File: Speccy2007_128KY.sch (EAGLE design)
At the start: 121 parts, among them J1 0, J2 0, X1 5V, X2 SCART-F, X3 PS/2 KB, X3P KB, X4 SD Card, X5 ByteBlaster, X6 AVRISP

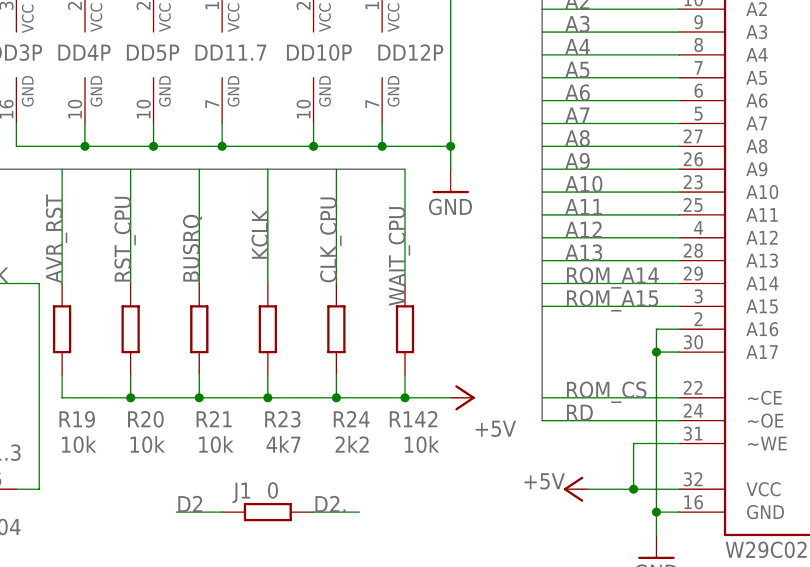
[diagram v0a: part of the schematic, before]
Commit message: t2
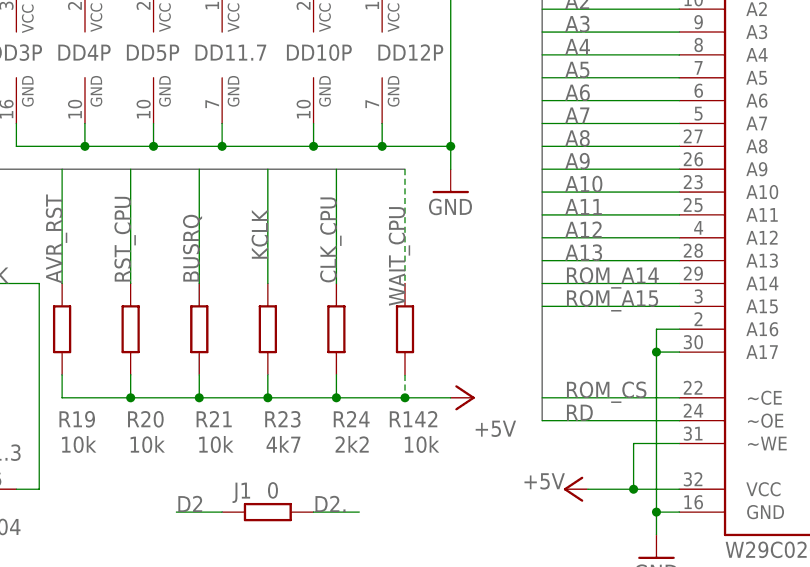
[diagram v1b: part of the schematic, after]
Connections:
- net N$16 renamed CDDAT3
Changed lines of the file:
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@@
 <grid distance="100" unitdist="mil" unit="mil" style="lines" multiple="1" display="yes" altdistance="0.01" altunitdist="inch" altunit="inch"/>
 <layers>
-<layer number="1" name="Top" color="4" fill="1" visible="yes" active="no"/>
-<layer number="2" name="Route2" color="1" fill="3" visible="yes" active="no"/>
-<layer number="3" name="Route3" color="4" fill="3" visible="yes" active="no"/>
-<layer number="4" name="Route4" color="1" fill="4" visible="yes" active="no"/>
-<layer number="5" name="Route5" color="4" fill="4" visible="yes" active="no"/>
-<layer number="6" name="Route6" color="1" fill="8" visible="yes" active="no"/>
-<layer number="7" name="Route7" color="4" fill="8" visible="yes" active="no"/>
-<layer number="8" name="Route8" color="1" fill="2" visible="yes" active="no"/>
-<layer number="9" name="Route9" color="4" fill="2" visible="yes" active="no"/>
-<layer number="10" name="Route10" color="1" fill="7" visible="yes" active="no"/>
-<layer number="11" name="Route11" color="4" fill="7" visible="yes" active="no"/>
-<layer number="12" name="Route12" color="1" fill="5" visible="yes" active="no"/>
-<layer number="13" name="Route13" color="4" fill="5" visible="yes" active="no"/>
-<layer number="14" name="Route14" color="1" fill="6" visible="yes" active="no"/>
-<layer number="15" name="Route15" color="4" fill="6" visible="yes" active="no"/>
-<layer number="16" name="Bottom" color="1" fill="1" visible="yes" active="no"/>
-<layer number="17" name="Pads" color="2" fill="1" visible="yes" active="no"/>
-<layer number="18" name="Vias" color="2" fill="1" visible="yes" active="no"/>
-<layer number="19" name="Unrouted" color="6" fill="1" visible="yes" active="no"/>
-<layer number="20" name="Dimension" color="15" fill="1" visible="yes" active="no"/>
-<layer number="21" name="tPlace" color="7" fill="1" visible="yes" active="no"/>
-<layer number="22" name="bPlace" color="7" fill="1" visible="yes" active="no"/>
-<layer number="23" name="tOrigins" color="15" fill="1" visible="yes" active="no"/>
-<layer number="24" name="bOrigins" color="15" fill="1" visible="yes" active="no"/>
-<layer number="25" name="tNames" color="7" fill="1" visible="yes" active="no"/>
-<layer number="26" name="bNames" color="7" fill="1" visible="yes" active="no"/>
-<layer number="27" name="tValues" color="7" fill="1" visible="yes" active="no"/>
-<layer number="28" name="bValues" color="7" fill="1" visible="yes" active="no"/>
+<layer number="1" name="Top" color="4" fill="1" visible="no" active="no"/>
+<layer number="2" name="Route2" color="1" fill="3" visible="no" active="no"/>
+<layer number="3" name="Route3" color="4" fill="3" visible="no" active="no"/>
+<layer number="4" name="Route4" color="1" fill="4" visible="no" active="no"/>
+<layer number="5" name="Route5" color="4" fill="4" visible="no" active="no"/>
+<layer number="6" name="Route6" color="1" fill="8" visible="no" active="no"/>
+<layer number="7" name="Route7" color="4" fill="8" visible="no" active="no"/>
+<layer number="8" name="Route8" color="1" fill="2" visible="no" active="no"/>
+<layer number="9" name="Route9" color="4" fill="2" visible="no" active="no"/>
+<layer number="10" name="Route10" color="1" fill="7" visible="no" active="no"/>
+<layer number="11" name="Route11" color="4" fill="7" visible="no" active="no"/>
+<layer number="12" name="Route12" color="1" fill="5" visible="no" active="no"/>
+<layer number="13" name="Route13" color="4" fill="5" visible="no" active="no"/>
+<layer number="14" name="Route14" color="1" fill="6" visible="no" active="no"/>
+<layer number="15" name="Route15" color="4" fill="6" visible="no" active="no"/>
+<layer number="16" name="Bottom" color="1" fill="1" visible="no" active="no"/>
+<layer number="17" name="Pads" color="2" fill="1" visible="no" active="no"/>
+<layer number="18" name="Vias" color="2" fill="1" visible="no" active="no"/>
+<layer number="19" name="Unrouted" color="6" fill="1" visible="no" active="no"/>
+<layer number="20" name="Dimension" color="15" fill="1" visible="no" active="no"/>
+<layer number="21" name="tPlace" color="7" fill="1" visible="no" active="no"/>
+<layer number="22" name="bPlace" color="7" fill="1" visible="no" active="no"/>
+<layer number="23" name="tOrigins" color="15" fill="1" visible="no" active="no"/>
+<layer number="24" name="bOrigins" color="15" fill="1" visible="no" active="no"/>
+<layer number="25" name="tNames" color="7" fill="1" visible="no" active="no"/>
+<layer number="26" name="bNames" color="7" fill="1" visible="no" active="no"/>
+<layer number="27" name="tValues" color="7" fill="1" visible="no" active="no"/>
+<layer number="28" name="bValues" color="7" fill="1" visible="no" active="no"/>
 <layer number="29" name="tStop" color="7" fill="3" visible="no" active="no"/>
 <layer number="30" name="bStop" color="7" fill="6" visible="no" active="no"/>
@@
 <layer number="35" name="tGlue" color="7" fill="4" visible="no" active="no"/>
 <layer number="36" name="bGlue" color="7" fill="5" visible="no" active="no"/>
-<layer number="37" name="tTest" color="7" fill="1" visible="yes" active="no"/>
-<layer number="38" name="bTest" color="7" fill="1" visible="yes" active="no"/>
+<layer number="37" name="tTest" color="7" fill="1" visible="no" active="no"/>
+<layer number="38" name="bTest" color="7" fill="1" visible="no" active="no"/>
 <layer number="39" name="tKeepout" color="4" fill="11" visible="no" active="no"/>
 <layer number="40" name="bKeepout" color="1" fill="11" visible="no" active="no"/>
@@
 <layer number="44" name="Drills" color="7" fill="1" visible="no" active="no"/>
 <layer number="45" name="Holes" color="7" fill="1" visible="no" active="no"/>
-<layer number="46" name="Milling" color="3" fill="1" visible="yes" active="no"/>
-<layer number="47" name="Measures" color="7" fill="1" visible="yes" active="no"/>
-<layer number="48" name="Document" color="7" fill="1" visible="yes" active="no"/>
-<layer number="49" name="Reference" color="7" fill="1" visible="yes" active="no"/>
-<layer number="50" name="dxf" color="7" fill="1" visible="yes" active="no"/>
-<layer number="51" name="tDocu" color="7" fill="1" visible="yes" active="no"/>
-<layer number="52" name="bDocu" color="7" fill="1" visible="yes" active="no"/>
-<layer number="53" name="tGND_GNDA" color="7" fill="9" visible="yes" active="no"/>
-<layer number="54" name="bGND_GNDA" color="1" fill="9" visible="yes" active="no"/>
-<layer number="56" name="wert" color="7" fill="1" visible="yes" active="no"/>
-<layer number="57" name="tCAD" color="7" fill="1" visible="yes" active="no"/>
+<layer number="46" name="Milling" color="3" fill="1" visible="no" active="no"/>
+<layer number="47" name="Measures" color="7" fill="1" visible="no" active="no"/>
+<layer number="48" name="Document" color="7" fill="1" visible="no" active="no"/>
+<layer number="49" name="Reference" color="7" fill="1" visible="no" active="no"/>
+<layer number="50" name="dxf" color="7" fill="1" visible="no" active="no"/>
+<layer number="51" name="tDocu" color="7" fill="1" visible="no" active="no"/>
+<layer number="52" name="bDocu" color="7" fill="1" visible="no" active="no"/>
+<layer number="53" name="tGND_GNDA" color="7" fill="9" visible="no" active="no"/>
+<layer number="54" name="bGND_GNDA" color="1" fill="9" visible="no" active="no"/>
+<layer number="56" name="wert" color="7" fill="1" visible="no" active="no"/>
+<layer number="57" name="tCAD" color="7" fill="1" visible="no" active="no"/>
 <layer number="90" name="Modules" color="5" fill="1" visible="yes" active="yes"/>
 <layer number="91" name="Nets" color="2" fill="1" visible="yes" active="yes"/>
@@
 <segment>
 <pinref part="R142" gate="G$1" pin="2"/>
-<wire x1="121.92" y1="53.34" x2="121.92" y2="40.64" width="0.1524" layer="91"/>
+<wire x1="121.92" y1="53.34" x2="121.92" y2="40.64" width="0.1524" layer="91" style="shortdash"/>
 <label x="121.92" y="38.1" size="1.778" layer="95" rot="R90"/>
 </segment>
@@
 <junction x="114.3" y="27.94"/>
 <pinref part="R142" gate="G$1" pin="1"/>
-<wire x1="121.92" y1="30.48" x2="121.92" y2="27.94" width="0.1524" layer="91"/>
+<wire x1="121.92" y1="30.48" x2="121.92" y2="27.94" width="0.1524" layer="91" style="shortdash"/>
 <junction x="121.92" y="27.94"/>
 </segment>
@@
 </segment>
 </net>
-<net name="N$16" class="0">
+<net name="CDDAT3" class="0">
 <segment>
 <pinref part="X4" gate="G$1" pin="CD/DAT3/CS"/>
